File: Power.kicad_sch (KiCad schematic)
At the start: 20 parts, among them IC2 TPS563209DDCR, U5 IC MCU 32BIT 1MB FLASH 64LQFP

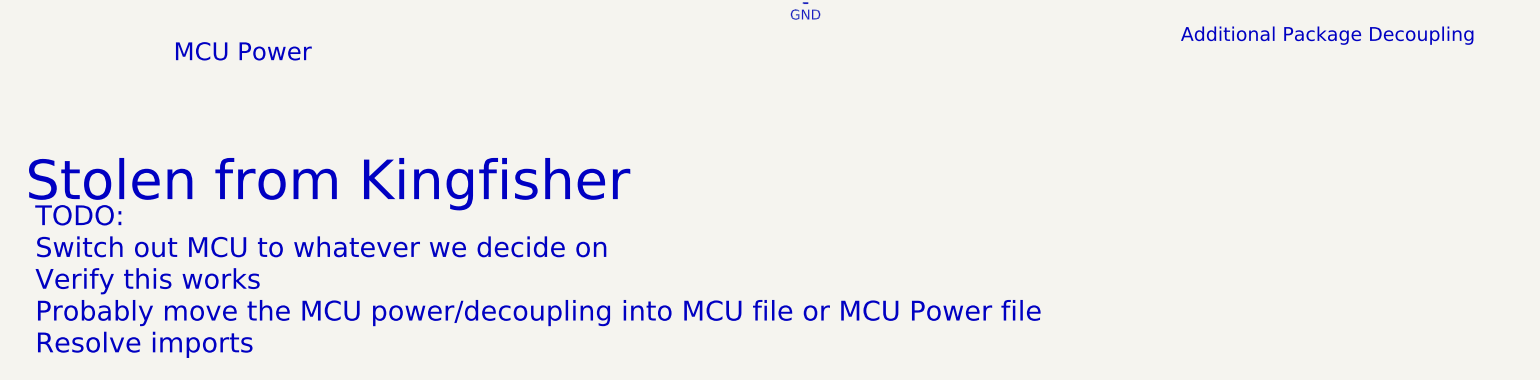
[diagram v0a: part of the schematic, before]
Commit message: Revert "Temporary save if I accidentally bust something"
This reverts commit 974f20a02fde00668d4b3d45f60811623d130148.
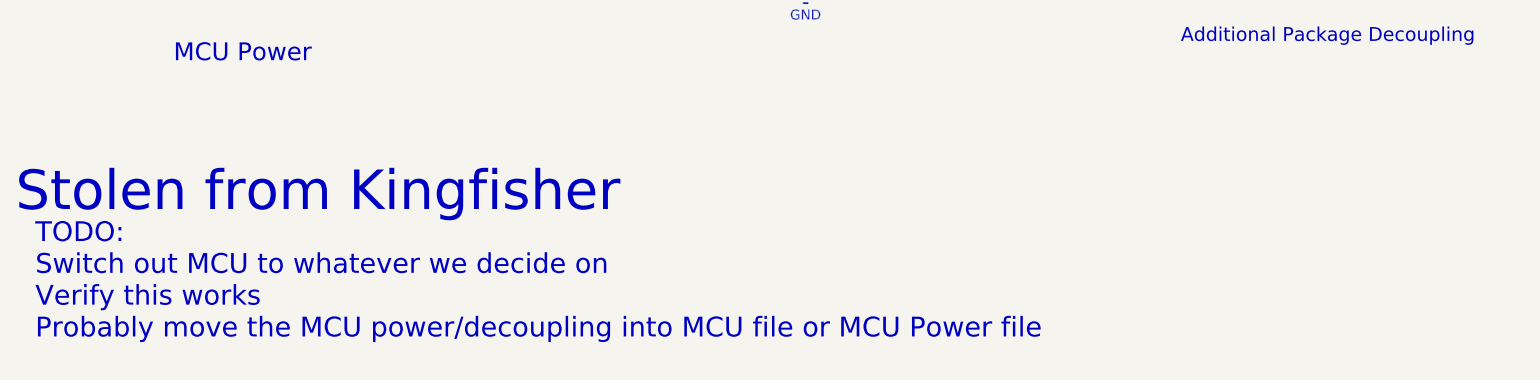
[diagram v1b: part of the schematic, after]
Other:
- note added: "TODO: Switch out MCU to whatever we decide on Verify this works Probably move the MCU power/decoupling into MCU file or MCU Power file"
- note removed: "TODO: Switch out MCU to whatever we decide on Verify this works Probably move the MCU power/decoupling into MCU file or MCU Power file Resolve imports"
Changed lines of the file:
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@@
 	(text "Stolen from Kingfisher\n"
 		(exclude_from_sim no)
-		(at 21.59 171.45 0)
+		(at 20.32 172.72 0)
 		(effects
 			(font
@@
 		)
 	)
-	(text "TODO:\nSwitch out MCU to whatever we decide on\nVerify this works\nProbably move the MCU power/decoupling into MCU file or MCU Power file\nResolve imports"
+	(text "TODO:\nSwitch out MCU to whatever we decide on\nVerify this works\nProbably move the MCU power/decoupling into MCU file or MCU Power file\n"
 		(exclude_from_sim no)
 		(at 22.86 184.15 0)

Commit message: Initial library setup
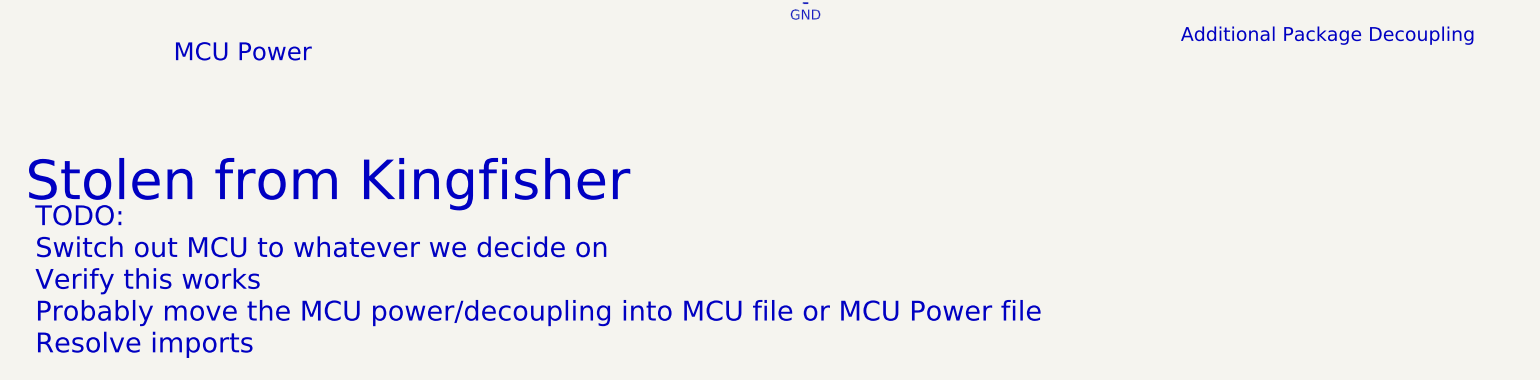
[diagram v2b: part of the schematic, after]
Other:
- note added: "TODO: Switch out MCU to whatever we decide on Verify this works Probably move the MCU power/decoupling into MCU file or MCU Power file Resolve imports"
- note removed: "TODO: Switch out MCU to whatever we decide on Verify this works Probably move the MCU power/decoupling into MCU file or MCU Power file"
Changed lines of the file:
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@@
 	(text "Stolen from Kingfisher\n"
 		(exclude_from_sim no)
-		(at 20.32 172.72 0)
+		(at 21.59 171.45 0)
 		(effects
 			(font
@@
 		)
 	)
-	(text "TODO:\nSwitch out MCU to whatever we decide on\nVerify this works\nProbably move the MCU power/decoupling into MCU file or MCU Power file\n"
+	(text "TODO:\nSwitch out MCU to whatever we decide on\nVerify this works\nProbably move the MCU power/decoupling into MCU file or MCU Power file\nResolve imports"
 		(exclude_from_sim no)
 		(at 22.86 184.15 0)
